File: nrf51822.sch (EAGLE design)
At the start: 5 parts

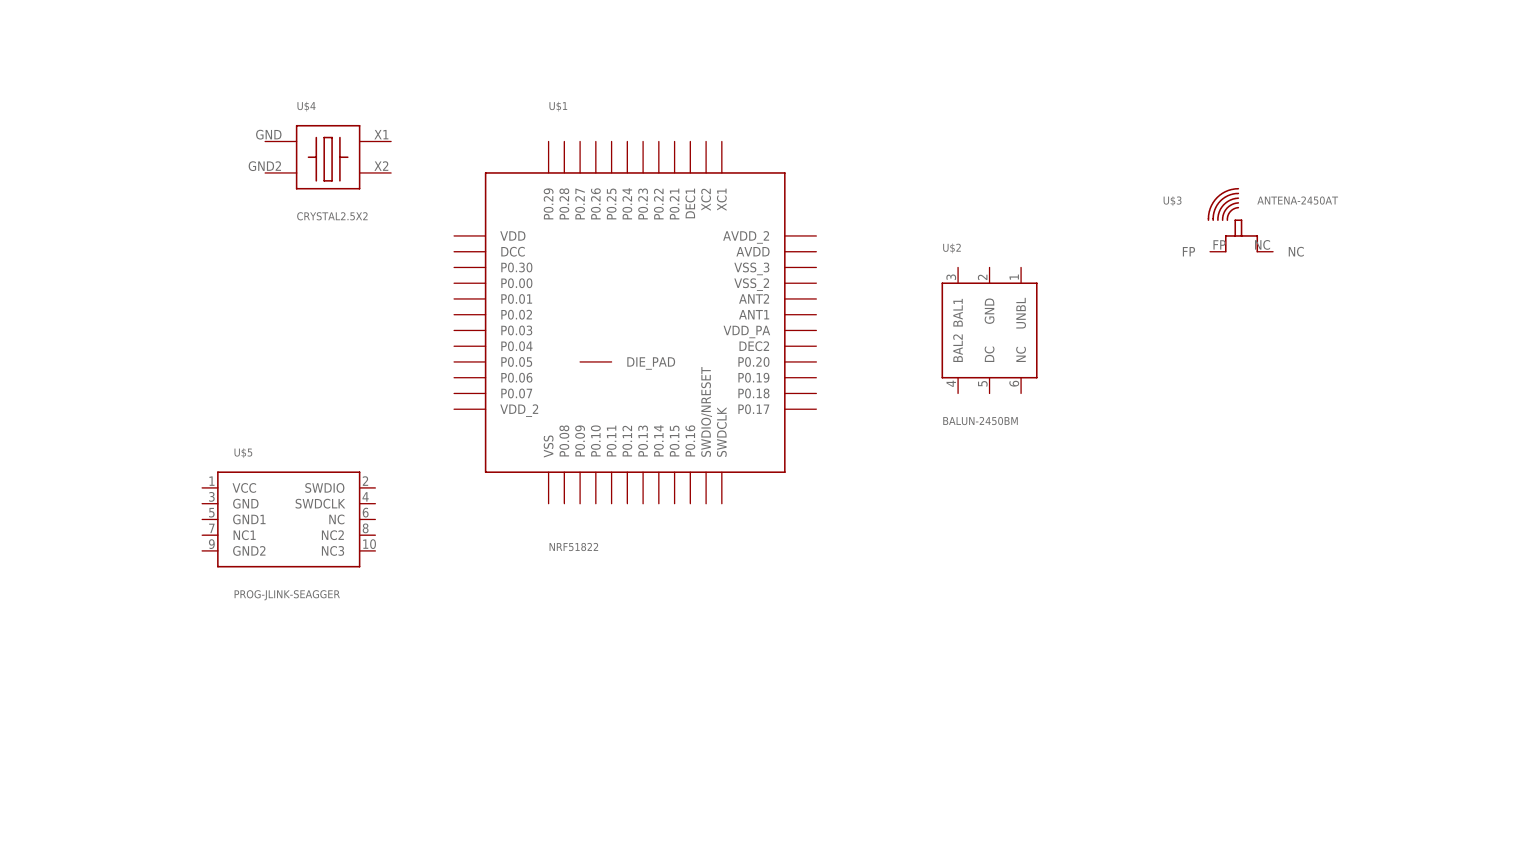
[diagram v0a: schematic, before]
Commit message: a few connectons
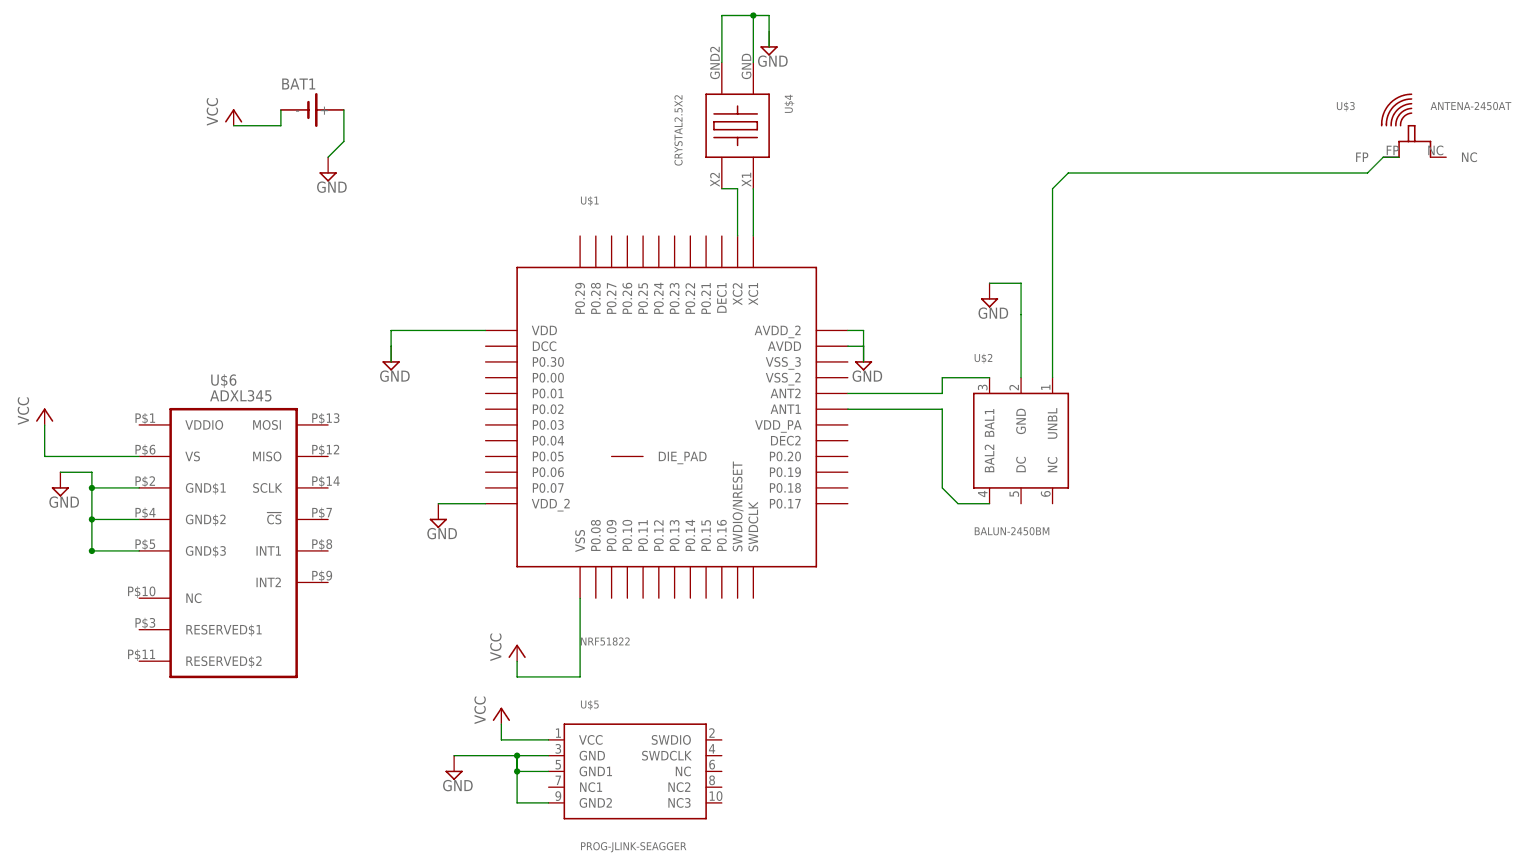
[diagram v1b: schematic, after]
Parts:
- added BAT1: (no value), sn2032:SN2032
- added U$6: ADXL345, adxl345:ADXL345
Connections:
- new net GND: BAT1.+, U$1.VDD, U$1.VDD_2, U$2.GND, U$5.GND, U$5.GND1, U$5.GND2, U$6.GND$1, U$6.GND$2, U$6.GND$3
- new net N$1: U$1.XC2, U$4.X2
- new net N$10: U$1.AVDD, U$1.AVDD_2
- new net N$12: U$4.GND, U$4.GND2
- new net N$2: U$1.XC1, U$4.X1
- new net N$6: U$1.ANT2, U$2.BAL1
- new net N$7: U$1.ANT1, U$2.BAL2
- new net N$8: U$2.UNBL, U$3.FP
- new net VCC: BAT1.-, U$1.VSS, U$5.VCC, U$6.VS
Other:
- moved on the sheet: U$1, U$2, U$3, U$4, U$5
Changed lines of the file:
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@@
 <part name="U$4" library="NordicSemi" deviceset="CRYSTAL2.5X2" device=""/>
 <part name="U$5" library="NordicSemi" deviceset="PROG-JLINK-SEAGGER" device=""/>
+<part name="U$6" library="adxl345" deviceset="ADXL345" device=""/>
+<part name="BAT1" library="sn2032" deviceset="SN2032" device=""/>
+<part name="SUPPLY1" library="supply2" deviceset="GND" device=""/>
+<part name="SUPPLY2" library="supply2" deviceset="GND" device=""/>
+<part name="SUPPLY3" library="supply2" deviceset="GND" device=""/>
+<part name="SUPPLY5" library="supply2" deviceset="GND" device=""/>
+<part name="SUPPLY6" library="supply2" deviceset="GND" device=""/>
+<part name="P+1" library="supply1" deviceset="VCC" device=""/>
+<part name="P+2" library="supply1" deviceset="VCC" device=""/>
+<part name="P+3" library="supply1" deviceset="VCC" device=""/>
+<part name="P+5" library="supply1" deviceset="VCC" device=""/>
+<part name="SUPPLY7" library="supply2" deviceset="GND" device=""/>
+<part name="SUPPLY8" library="supply2" deviceset="GND" device=""/>
+<part name="SUPPLY9" library="supply2" deviceset="GND" device=""/>
 </parts>
 <sheets>
@@
 </plain>
 <instances>
-<instance part="U$1" gate="G$1" x="38.1" y="22.86"/>
-<instance part="U$2" gate="G$1" x="121.92" y="48.26"/>
-<instance part="U$3" gate="G$1" x="160.02" y="60.96"/>
-<instance part="U$4" gate="G$1" x="15.24" y="76.2"/>
-<instance part="U$5" gate="G$1" x="10.16" y="17.78"/>
+<instance part="U$1" gate="G$1" x="43.18" y="7.62"/>
+<instance part="U$2" gate="G$1" x="127" y="30.48"/>
+<instance part="U$3" gate="G$1" x="187.96" y="76.2"/>
+<instance part="U$4" gate="G$1" x="81.28" y="81.28" rot="R270"/>
+<instance part="U$5" gate="G$1" x="66.04" y="-22.86"/>
+<instance part="U$6" gate="G$1" x="0" y="15.24"/>
+<instance part="BAT1" gate="1" x="12.7" y="83.82"/>
+<instance part="SUPPLY1" gate="GND" x="15.24" y="73.66"/>
+<instance part="SUPPLY2" gate="GND" x="121.92" y="53.34"/>
+<instance part="SUPPLY3" gate="GND" x="35.56" y="-22.86"/>
+<instance part="SUPPLY5" gate="GND" x="33.02" y="17.78"/>
+<instance part="SUPPLY6" gate="GND" x="101.6" y="43.18"/>
+<instance part="P+1" gate="VCC" x="0" y="83.82"/>
+<instance part="P+2" gate="VCC" x="-30.48" y="35.56"/>
+<instance part="P+3" gate="VCC" x="45.72" y="-2.54"/>
+<instance part="P+5" gate="VCC" x="43.18" y="-12.7"/>
+<instance part="SUPPLY7" gate="GND" x="25.4" y="43.18"/>
+<instance part="SUPPLY8" gate="GND" x="86.36" y="93.98"/>
+<instance part="SUPPLY9" gate="GND" x="-27.94" y="22.86"/>
 </instances>
 <busses>
 </busses>
 <nets>
+<net name="N$1" class="0">
+<segment>
+<pinref part="U$4" gate="G$1" pin="X2"/>
+<pinref part="U$1" gate="G$1" pin="XC2"/>
+<wire x1="78.74" y1="71.12" x2="81.28" y2="71.12" width="0.1524" layer="91"/>
+<wire x1="81.28" y1="71.12" x2="81.28" y2="63.5" width="0.1524" layer="91"/>
+</segment>
+</net>
+<net name="N$2" class="0">
+<segment>
+<pinref part="U$4" gate="G$1" pin="X1"/>
+<pinref part="U$1" gate="G$1" pin="XC1"/>
+<wire x1="83.82" y1="71.12" x2="83.82" y2="63.5" width="0.1524" layer="91"/>
+</segment>
+</net>
+<net name="N$6" class="0">
+<segment>
+<pinref part="U$2" gate="G$1" pin="BAL1"/>
+<pinref part="U$1" gate="G$1" pin="ANT2"/>
+<wire x1="121.92" y1="40.64" x2="114.3" y2="40.64" width="0.1524" layer="91"/>
+<wire x1="114.3" y1="40.64" x2="114.3" y2="38.1" width="0.1524" layer="91"/>
+<wire x1="114.3" y1="38.1" x2="99.06" y2="38.1" width="0.1524" layer="91"/>
+</segment>
+</net>
+<net name="N$7" class="0">
+<segment>
+<pinref part="U$2" gate="G$1" pin="BAL2"/>
+<wire x1="121.92" y1="20.32" x2="116.84" y2="20.32" width="0.1524" layer="91"/>
+<wire x1="116.84" y1="20.32" x2="114.3" y2="22.86" width="0.1524" layer="91"/>
+<wire x1="114.3" y1="22.86" x2="114.3" y2="35.56" width="0.1524" layer="91"/>
+<pinref part="U$1" gate="G$1" pin="ANT1"/>
+<wire x1="114.3" y1="35.56" x2="99.06" y2="35.56" width="0.1524" layer="91"/>
+</segment>
+</net>
+<net name="N$8" class="0">
+<segment>
+<pinref part="U$2" gate="G$1" pin="UNBL"/>
+<wire x1="132.08" y1="40.64" x2="132.08" y2="71.12" width="0.1524" layer="91"/>
+<wire x1="132.08" y1="71.12" x2="134.62" y2="73.66" width="0.1524" layer="91"/>
+<wire x1="134.62" y1="73.66" x2="182.88" y2="73.66" width="0.1524" layer="91"/>
+<wire x1="182.88" y1="73.66" x2="185.42" y2="76.2" width="0.1524" layer="91"/>
+<pinref part="U$3" gate="G$1" pin="FP"/>
+<wire x1="185.42" y1="76.2" x2="187.96" y2="76.2" width="0.1524" layer="91"/>
+</segment>
+</net>
+<net name="GND" class="0">
+<segment>
+<pinref part="BAT1" gate="1" pin="+"/>
+<wire x1="17.78" y1="83.82" x2="17.78" y2="78.74" width="0.1524" layer="91"/>
+<wire x1="17.78" y1="78.74" x2="15.24" y2="76.2" width="0.1524" layer="91"/>
+<pinref part="SUPPLY1" gate="GND" pin="GND"/>
+</segment>
+<segment>
+<pinref part="U$6" gate="G$1" pin="GND$1"/>
+<wire x1="-15.24" y1="22.86" x2="-22.86" y2="22.86" width="0.1524" layer="91"/>
+<wire x1="-22.86" y1="22.86" x2="-22.86" y2="25.4" width="0.1524" layer="91"/>
+<pinref part="SUPPLY9" gate="GND" pin="GND"/>
+<wire x1="-22.86" y1="25.4" x2="-27.94" y2="25.4" width="0.1524" layer="91"/>
+<pinref part="U$6" gate="G$1" pin="GND$3"/>
+<wire x1="-15.24" y1="12.7" x2="-22.86" y2="12.7" width="0.1524" layer="91"/>
+<wire x1="-22.86" y1="12.7" x2="-22.86" y2="17.78" width="0.1524" layer="91"/>
+<pinref part="U$6" gate="G$1" pin="GND$2"/>
+<wire x1="-22.86" y1="17.78" x2="-22.86" y2="22.86" width="0.1524" layer="91"/>
+<wire x1="-15.24" y1="17.78" x2="-22.86" y2="17.78" width="0.1524" layer="91"/>
+<junction x="-22.86" y="22.86"/>
+<junction x="-22.86" y="17.78"/>
+<junction x="-22.86" y="12.7"/>
+</segment>
+<segment>
+<pinref part="U$5" gate="G$1" pin="GND"/>
+<pinref part="SUPPLY3" gate="GND" pin="GND"/>
+<wire x1="50.8" y1="-20.32" x2="45.72" y2="-20.32" width="0.1524" layer="91"/>
+<pinref part="U$5" gate="G$1" pin="GND1"/>
+<wire x1="45.72" y1="-20.32" x2="35.56" y2="-20.32" width="0.1524" layer="91"/>
+<wire x1="50.8" y1="-22.86" x2="45.72" y2="-22.86" width="0.1524" layer="91"/>
+<wire x1="45.72" y1="-22.86" x2="45.72" y2="-20.32" width="0.1524" layer="91"/>
+<junction x="45.72" y="-20.32"/>
+<pinref part="U$5" gate="G$1" pin="GND2"/>
+<wire x1="50.8" y1="-27.94" x2="45.72" y2="-27.94" width="0.1524" layer="91"/>
+<wire x1="45.72" y1="-27.94" x2="45.72" y2="-22.86" width="0.1524" layer="91"/>
+<junction x="45.72" y="-22.86"/>
+<wire x1="45.72" y1="-22.86" x2="45.72" y2="-20.32" width="0.1524" layer="91"/>
+</segment>
+<segment>
+<pinref part="U$1" gate="G$1" pin="VDD"/>
+<wire x1="40.64" y1="48.26" x2="25.4" y2="48.26" width="0.1524" layer="91"/>
+<wire x1="25.4" y1="48.26" x2="25.4" y2="45.72" width="0.1524" layer="91"/>
+<pinref part="SUPPLY7" gate="GND" pin="GND"/>
+<wire x1="25.4" y1="43.18" x2="25.4" y2="45.72" width="0.1524" layer="91"/>
+</segment>
+<segment>
+<pinref part="U$1" gate="G$1" pin="VDD_2"/>
+<pinref part="SUPPLY5" gate="GND" pin="GND"/>
+<wire x1="40.64" y1="20.32" x2="33.02" y2="20.32" width="0.1524" layer="91"/>
+</segment>
+<segment>
+<pinref part="U$2" gate="G$1" pin="GND"/>
+<pinref part="SUPPLY2" gate="GND" pin="GND"/>
+<wire x1="127" y1="40.64" x2="127" y2="50.8" width="0.1524" layer="91"/>
+<wire x1="127" y1="50.8" x2="127" y2="55.88" width="0.1524" layer="91"/>
+<wire x1="127" y1="55.88" x2="121.92" y2="55.88" width="0.1524" layer="91"/>
+</segment>
+</net>
+<net name="VCC" class="0">
+<segment>
+<pinref part="P+1" gate="VCC" pin="VCC"/>
+<pinref part="BAT1" gate="1" pin="-"/>
+<wire x1="0" y1="81.28" x2="7.62" y2="81.28" width="0.1524" layer="91"/>
+<wire x1="7.62" y1="81.28" x2="7.62" y2="83.82" width="0.1524" layer="91"/>
+</segment>
+<segment>
+<pinref part="U$5" gate="G$1" pin="VCC"/>
+<wire x1="50.8" y1="-17.78" x2="43.18" y2="-17.78" width="0.1524" layer="91"/>
+<pinref part="P+5" gate="VCC" pin="VCC"/>
+<wire x1="43.18" y1="-17.78" x2="43.18" y2="-15.24" width="0.1524" layer="91"/>
+</segment>
+<segment>
+<pinref part="U$6" gate="G$1" pin="VS"/>
+<wire x1="-15.24" y1="27.94" x2="-30.48" y2="27.94" width="0.1524" layer="91"/>
+<pinref part="P+2" gate="VCC" pin="VCC"/>
+<wire x1="-30.48" y1="27.94" x2="-30.48" y2="33.02" width="0.1524" layer="91"/>
+</segment>
+<segment>
+<pinref part="U$1" gate="G$1" pin="VSS"/>
+<wire x1="55.88" y1="5.08" x2="55.88" y2="-7.62" width="0.1524" layer="91"/>
+<wire x1="55.88" y1="-7.62" x2="45.72" y2="-7.62" width="0.1524" layer="91"/>
+<pinref part="P+3" gate="VCC" pin="VCC"/>
+<wire x1="45.72" y1="-7.62" x2="45.72" y2="-5.08" width="0.1524" layer="91"/>
+</segment>
+</net>
+<net name="N$10" class="0">
+<segment>
+<pinref part="U$1" gate="G$1" pin="AVDD_2"/>
+<wire x1="99.06" y1="48.26" x2="101.6" y2="48.26" width="0.1524" layer="91"/>
+<wire x1="101.6" y1="48.26" x2="101.6" y2="45.72" width="0.1524" layer="91"/>
+<pinref part="U$1" gate="G$1" pin="AVDD"/>
+<wire x1="101.6" y1="45.72" x2="101.6" y2="43.18" width="0.1524" layer="91"/>
+<wire x1="99.06" y1="45.72" x2="101.6" y2="45.72" width="0.1524" layer="91"/>
+</segment>
+</net>
+<net name="N$12" class="0">
+<segment>
+<pinref part="U$4" gate="G$1" pin="GND2"/>
+<wire x1="78.74" y1="91.44" x2="78.74" y2="99.06" width="0.1524" layer="91"/>
+<wire x1="78.74" y1="99.06" x2="83.82" y2="99.06" width="0.1524" layer="91"/>
+<wire x1="83.82" y1="99.06" x2="86.36" y2="99.06" width="0.1524" layer="91"/>
+<wire x1="86.36" y1="99.06" x2="86.36" y2="93.98" width="0.1524" layer="91"/>
+<pinref part="U$4" gate="G$1" pin="GND"/>
+<wire x1="83.82" y1="91.44" x2="83.82" y2="99.06" width="0.1524" layer="91"/>
+<junction x="83.82" y="99.06"/>
+</segment>
+</net>
 </nets>
 </sheet>
